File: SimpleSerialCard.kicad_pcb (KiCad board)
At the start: 4 copper layers, 98.8 x 85.1 mm, 25 parts, among them J1 IRQ ENABLE, J2 RS-232 OUT, P1 A2Bus, U1 74HCT245, U2 28C256, U3 1.8432M, U4 SSCGLU, U5 W65C51NxP, U6 MAX3232, U7 MAX3232

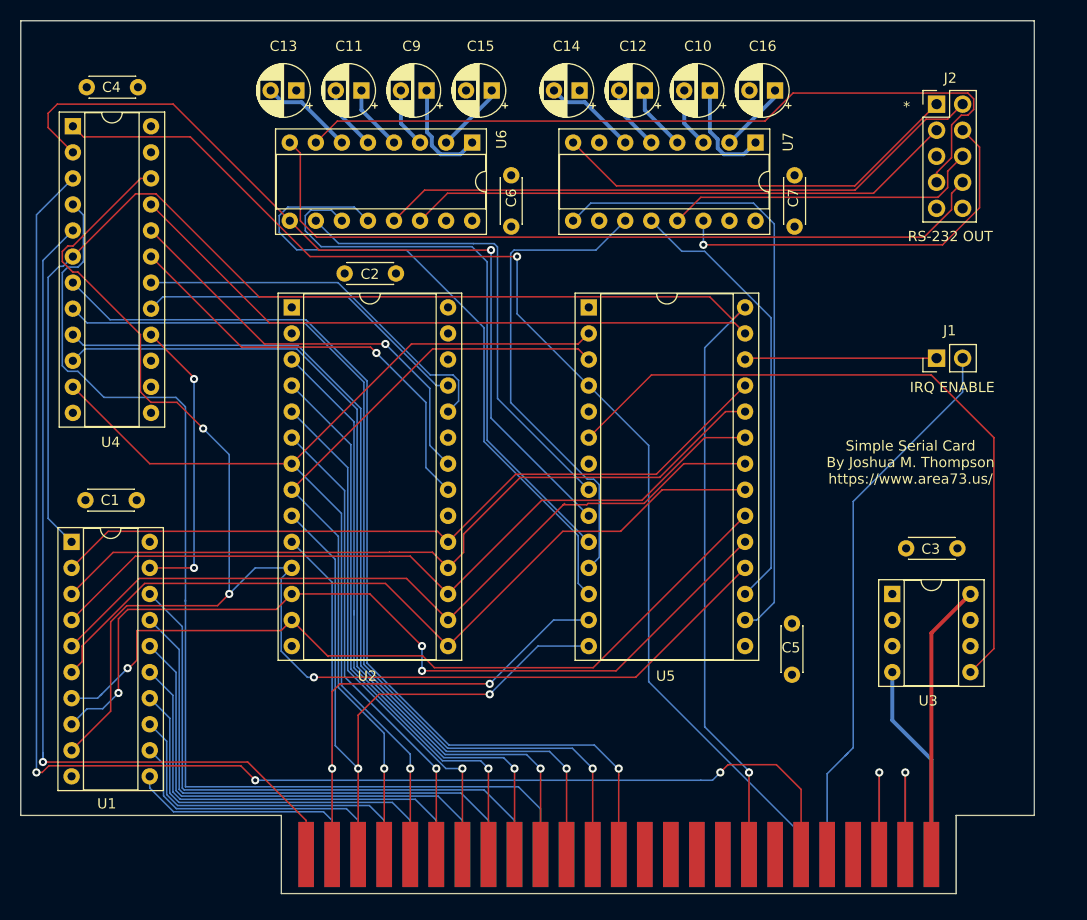
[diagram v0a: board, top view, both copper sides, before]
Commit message: reroute everything
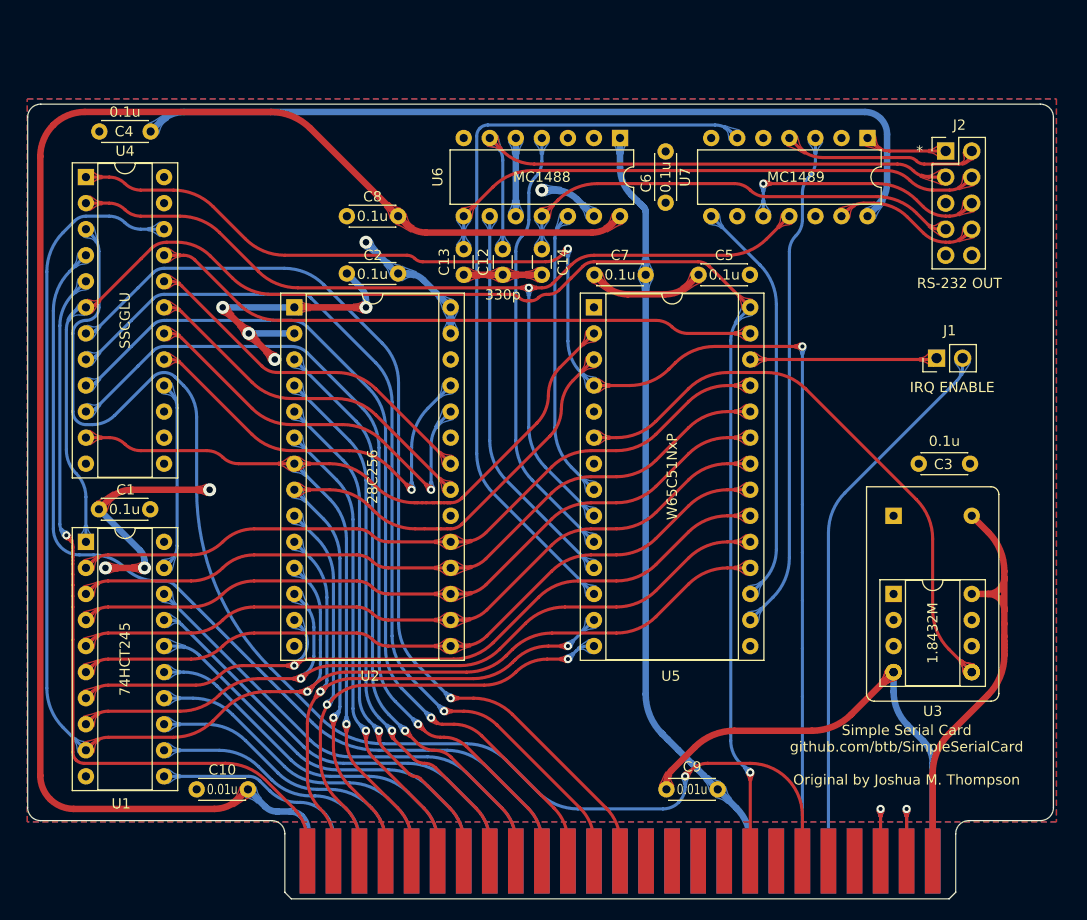
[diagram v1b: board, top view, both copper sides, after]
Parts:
- removed C11, C15, C16: 1u, Capacitor_THT:CP_Radial_D5.0mm_P2.50mm
- added ALT_U3: 1.8432M, Oscillator:Oscillator_DIP-14, F.Cu at (186.7, 90.2)
- added C8: 0.1u, Capacitor_THT:C_Disc_D4.3mm_W1.9mm_P5.00mm, F.Cu at (138.4, 61.0)
- C10, C9: value 1u -> 0.01u; footprint Capacitor_THT:CP_Radial_D5.0mm_P2.50mm -> Capacitor_THT:C_Disc_D4.3mm_W1.9mm_P5.00mm
- C12, C13, C14: value 1u -> 330p; footprint Capacitor_THT:CP_Radial_D5.0mm_P2.50mm -> Capacitor_THT:C_Disc_D3.0mm_W1.6mm_P2.50mm
- U6: value MAX3232 -> MC1488; footprint Package_DIP:DIP-16_W7.62mm_Socket -> Package_DIP:DIP-14_W7.62mm
- U7: value MAX3232 -> MC1489; footprint Package_DIP:DIP-16_W7.62mm_Socket -> Package_DIP:DIP-14_W7.62mm
- moved C10 81.7 mm to (123.7, 116.8)
- moved C9 72.0 mm to (164.5, 116.8), turned to 0 degrees
- moved C5 39.2 mm to (172.7, 66.7), turned to 180 degrees
- moved C13 22.5 mm to (144.8, 64.2), turned to -90 degrees
- moved C12 20.8 mm to (148.6, 64.2), turned to -90 degrees
- moved C7 20.1 mm to (157.5, 66.7), turned to 0 degrees
- moved C14 15.9 mm to (152.4, 64.2), turned to -90 degrees
- moved C6 15.2 mm to (164.5, 59.6)
- moved U6 14.4 mm to (160.0, 53.3)
- moved U7 10.9 mm to (184.2, 53.3)
- moved C3 8.35 mm to (194.1, 85.1)
- moved U4 5.11 mm to (108.0, 57.1)
- moved J2 4.66 mm to (191.8, 54.6)
- moved C4 4.49 mm to (114.3, 52.7)
- moved C1 1.59 mm to (114.2, 89.5)
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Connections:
- net R~W renamed R~{W}
- net ~DEVSEL renamed ~{DEVSEL}
- net ~IOSEL renamed ~{IOSEL}
- net ~IOSTRB renamed ~{IOSTRB}
- net ~IRQ renamed ~{IRQ}
- net ~LATCHCE renamed ~{LATCHCE}
- net ~RES renamed ~{RES}
- net ~ROMOE renamed ~{ROMOE}
- C10 pad 1: Net-(C10-Pad1) -> +12V
- C10 pad 2: Net-(C10-Pad2) -> GND
- C12 pad 2: Net-(C12-Pad2) -> GND
- C13 pad 1: GND -> Net-(C13-Pad1)
- C13 pad 2: Net-(C13-Pad2) -> GND
- C14 pad 1: GND -> Net-(C14-Pad1)
- C14 pad 2: Net-(C14-Pad2) -> GND
- C7 pad 1: +5V -> GND
- C7 pad 2: GND -> -12V
- C9 pad 1: Net-(C9-Pad1) -> GND
- C9 pad 2: Net-(C9-Pad2) -> -12V
- J2 pad 3: Net-(J2-Pad3) -> Net-(C12-Pad1)
- J2 pad 4: Net-(J2-Pad4) -> Net-(C13-Pad1)
- J2 pad 7: Net-(J2-Pad7) -> Net-(C14-Pad1)
- J2 pad 9: (no net) -> unconnected-(J2-Pad9)
- P1 pad 14: (no net) -> unconnected-(P1-Pad14)
- P1 pad 15: (no net) -> unconnected-(P1-Pad15)
- P1 pad 16: (no net) -> unconnected-(P1-Pad16)
- P1 pad 17: (no net) -> unconnected-(P1-Pad17)
- P1 pad 19: (no net) -> unconnected-(P1-Pad19)
- P1 pad 21: (no net) -> unconnected-(P1-Pad21)
- P1 pad 22: (no net) -> unconnected-(P1-Pad22)
- P1 pad 29: (no net) -> unconnected-(P1-Pad29)
- P1 pad 32: (no net) -> unconnected-(P1-Pad32)
- P1 pad 33: (no net) -> -12V
- P1 pad 34: (no net) -> unconnected-(P1-Pad34)
- P1 pad 35: (no net) -> unconnected-(P1-Pad35)
- P1 pad 36: (no net) -> unconnected-(P1-Pad36)
- P1 pad 37: (no net) -> unconnected-(P1-Pad37)
- P1 pad 38: (no net) -> unconnected-(P1-Pad38)
- P1 pad 39: (no net) -> unconnected-(P1-Pad39)
- P1 pad 40: (no net) -> unconnected-(P1-Pad40)
- P1 pad 50: (no net) -> +12V
- U5 pad 5: (no net) -> unconnected-(U5-Pad5)
- U5 pad 7: (no net) -> unconnected-(U5-Pad7)
- U6 pad 1: Net-(C9-Pad1) -> -12V
- U6 pad 10: Net-(U5-Pad8) -> +5V
- U6 pad 11: Net-(U5-Pad10) -> Net-(C14-Pad1)
- U6 pad 12: Net-(U5-Pad12) -> Net-(U5-Pad8)
- U6 pad 13: Net-(J2-Pad2) -> +5V
- U6 pad 14: Net-(J2-Pad3) -> +12V
- U6 pad 2: Net-(C15-Pad1) -> unconnected-(U6-Pad2)
- U6 pad 3: Net-(C9-Pad2) -> unconnected-(U6-Pad3)
- U6 pad 4: Net-(C11-Pad1) -> Net-(U5-Pad10)
- U6 pad 5: Net-(C11-Pad2) -> +5V
- U6 pad 6: Net-(C13-Pad2) -> Net-(C12-Pad1)
- U6 pad 7: Net-(J2-Pad7) -> GND
- U6 pad 8: Net-(J2-Pad8) -> Net-(C13-Pad1)
- U6 pad 9: Net-(U4-Pad2) -> Net-(U5-Pad11)
- U7 pad 1: Net-(C10-Pad1) -> Net-(J2-Pad1)
- U7 pad 10: GND -> Net-(J2-Pad6)
- U7 pad 11: Net-(U5-Pad11) -> Net-(U4-Pad2)
- U7 pad 12: Net-(U5-Pad17) -> unconnected-(U7-Pad12)
- U7 pad 13: Net-(J2-Pad6) -> Net-(J2-Pad8)
- U7 pad 14: Net-(J2-Pad4) -> +5V
- U7 pad 2: Net-(C16-Pad1) -> unconnected-(U7-Pad2)
- U7 pad 3: Net-(C10-Pad2) -> Net-(U5-Pad16)
- U7 pad 4: Net-(C12-Pad1) -> Net-(J2-Pad2)
- U7 pad 5: Net-(C12-Pad2) -> unconnected-(U7-Pad5)
- U7 pad 6: Net-(C14-Pad2) -> Net-(U5-Pad12)
- U7 pad 7: (no net) -> GND
- U7 pad 8: Net-(J2-Pad1) -> Net-(U5-Pad17)
- U7 pad 9: Net-(U5-Pad16) -> unconnected-(U7-Pad9)
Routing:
- net +12V: track 0.00 -> 157.7 mm
- net +5V: track 27.0 -> 152.7 mm, vias 0 -> 2
- net GND: track 19.4 -> 118.0 mm, vias 0 -> 7
- net Net-(J2-Pad7): track 76.4 -> 0.00 mm
- net -12V: track 0.00 -> 75.1 mm
- net Net-(J2-Pad8): track 76.4 -> 14.7 mm
- net Net-(C13-Pad1): track 0.00 -> 55.2 mm
- net Net-(J2-Pad3): track 54.0 -> 0.00 mm
- net Net-(C12-Pad1): track 6.40 -> 56.9 mm
- net Net-(C14-Pad1): track 0.00 -> 44.9 mm
- net Net-(J2-Pad2): track 60.1 -> 19.2 mm
- net Net-(J2-Pad4): track 39.0 -> 0.00 mm, vias 1 -> 0
- net Net-(J2-Pad1): track 40.5 -> 8.04 mm
- net ~{DEVSEL}: track 108.4 -> 89.9 mm
- net Net-(U5-Pad8): track 46.1 -> 28.4 mm
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- added copper zone on F.Cu, net +5V
- added copper zone on B.Cu, net GND
- removed copper zone on In1.Cu, net +5V
- removed copper zone on In2.Cu, net GND
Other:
- board size 98.8 x 85.1 mm -> 100 x 77.5 mm
- copper layers 4 -> 2
- net class Default removed
- net class Power removed
- board text added: "Simple Serial Card github.com/btb/SimpleSerialCard Original by Joshua M. Thompson"
- board text removed: "Simple Serial Card By Joshua M. Thompson https://www.area73.us/"
